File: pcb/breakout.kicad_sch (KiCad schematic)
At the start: 1 part, among them J14 PINHD_1x8_Female

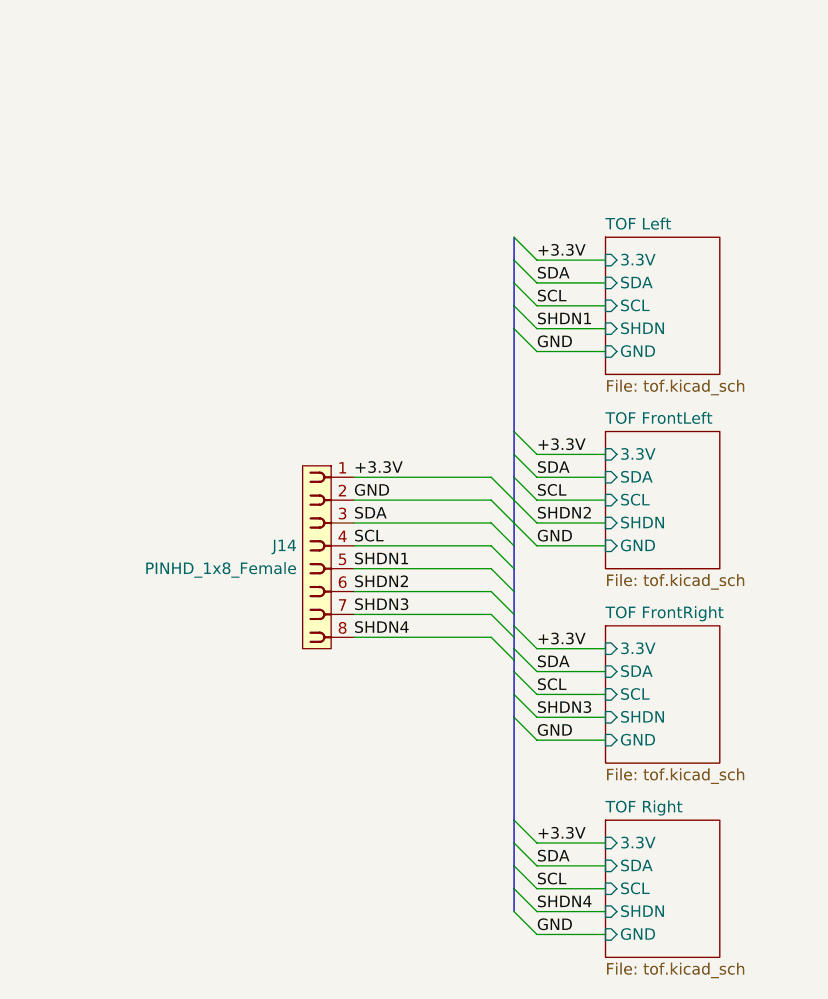
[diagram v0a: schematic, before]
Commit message: Add files via upload
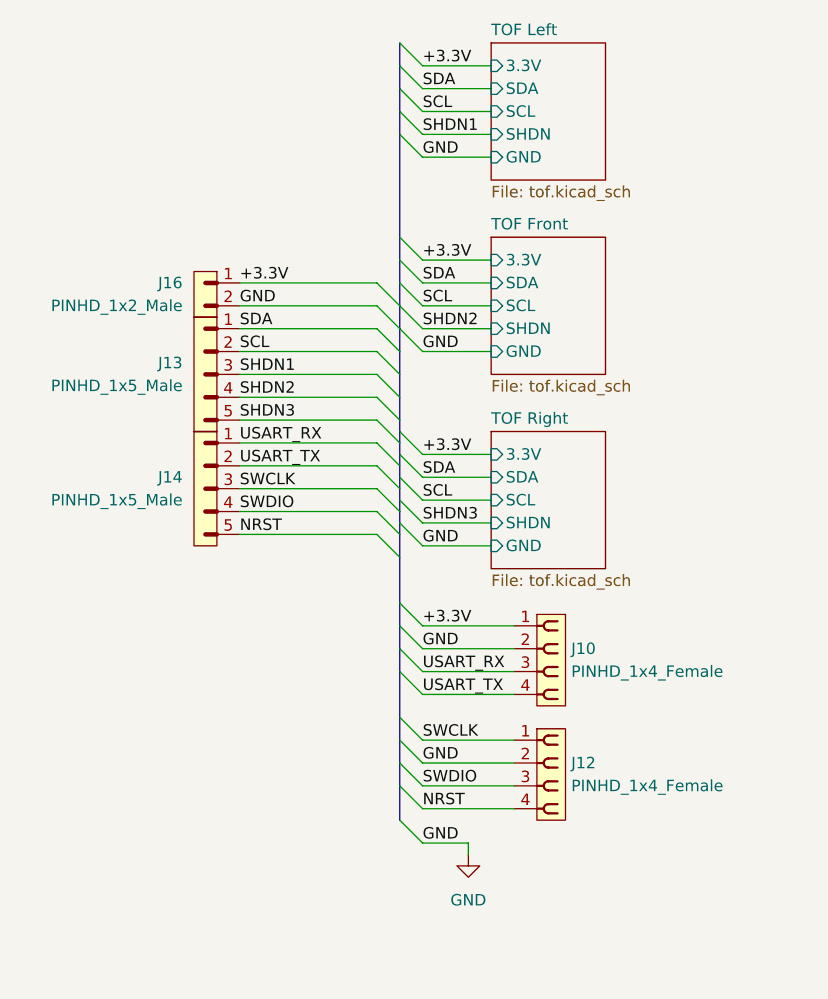
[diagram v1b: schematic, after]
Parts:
- removed J14: PINHD_1x8_Female, Connector_PinSocket_2.54mm:PinSocket_1x08_P2.54mm_Vertical, symbol PCM_SL_Pin_Headers:PINHD_1x8_Female
- added J10, J12: PINHD_1x4_Female, Connector_PinSocket_2.54mm:PinSocket_1x04_P2.54mm_Vertical, symbol PCM_SL_Pin_Headers:PINHD_1x4_Female
- added J13, J14: PINHD_1x5_Male, Connector_PinHeader_1.00mm:PinHeader_1x05_P1.00mm_Vertical, symbol PCM_SL_Pin_Headers:PINHD_1x5_Male
- added J16: PINHD_1x2_Male, Connector_PinHeader_2.54mm:PinHeader_1x02_P2.54mm_Vertical, symbol PCM_SL_Pin_Headers:PINHD_1x2_Male
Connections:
- net +3.3V: now also J10.1, J16.1
- net GND: now also J10.2, J12.2, J16.2
- net SCL: now also J13.2
- net SDA: now also J13.1
- net SHDN1: now also J13.3
- net SHDN2: now also J13.4
- net SHDN3: now also J13.5
- new net NRST: J12.4, J14.5
- new net SWCLK: J12.1, J14.3
- new net SWDIO: J12.3, J14.4
- new net USART_RX: J10.3, J14.1
- new net USART_TX: J10.4, J14.2
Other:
- sheet TOF FrontLeft renamed TOF Front
- removed sheet TOF FrontRight
